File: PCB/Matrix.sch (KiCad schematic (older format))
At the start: 167 parts

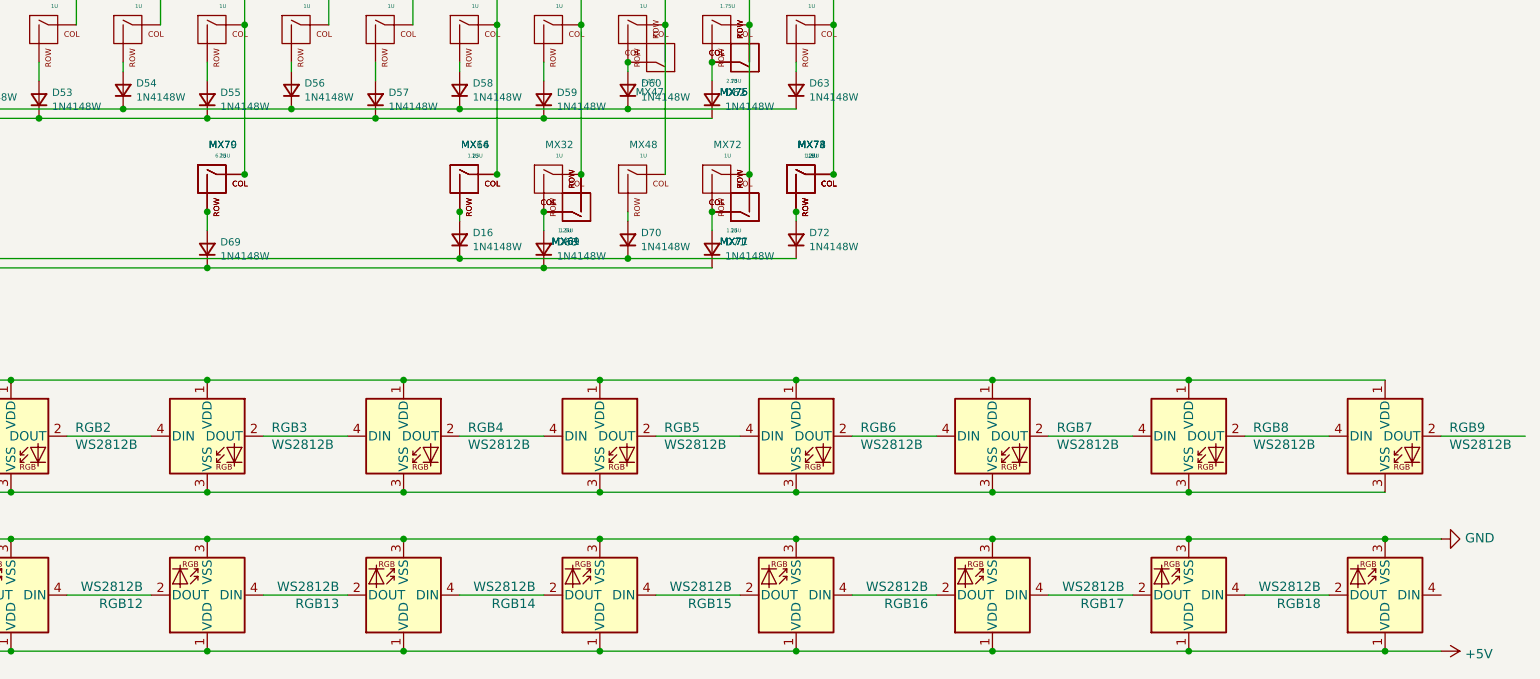
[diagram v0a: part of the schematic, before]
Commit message: PCB update
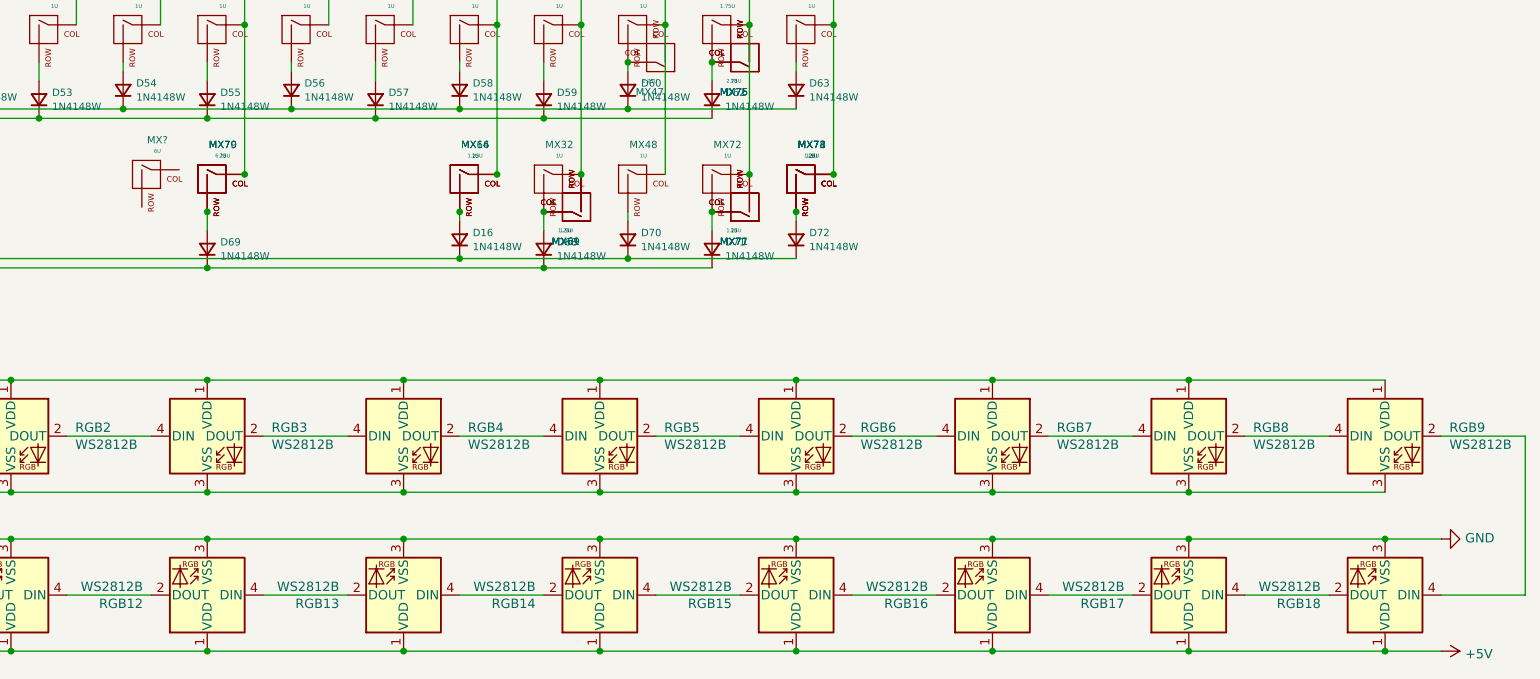
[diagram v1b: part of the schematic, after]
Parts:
- added MX?: 6U, MX_Solder_SawnsProjects:MXOnly-6U-ReversedStabilizers-NoLED, symbol random-keyboard-parts:MX-NoLED-MX_Alps_Hybrid
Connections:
- net at RGB9.2 (DOUT): now also RGB18.4 (DIN)
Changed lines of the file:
@@
 	5150 4550 5150 4600
 Connection ~ 5150 4550
+Wire Wire Line
+	10400 6600 10850 6600
+Wire Wire Line
+	10850 6600 10850 5750
+$Comp
+L random-keyboard-parts:MX-NoLED-MX_Alps_Hybrid MX?
+U 1 1 6342F4CC
+P 3500 4375
+F 0 "MX?" H 3533 4584 39  0000 C CNN
+F 1 "6U" H 3533 4525 20  0000 C CNN
+F 2 "MX_Solder_SawnsProjects:MXOnly-6U-ReversedStabilizers-NoLED" H 2875 4350 60  0001 C CNN
+F 3 "" H 2875 4350 60  0001 C CNN
+	1    3500 4375
+	1    0    0    -1
+$EndComp
 $EndSCHEMATC
